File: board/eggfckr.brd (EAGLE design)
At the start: 114 x 77.5 mm, 22 parts, among them U1 ATTINY85-20PU, U2 ATTINY85-20PU, U3 ATTINY85-20PU, U4 ATTINY85-20PU

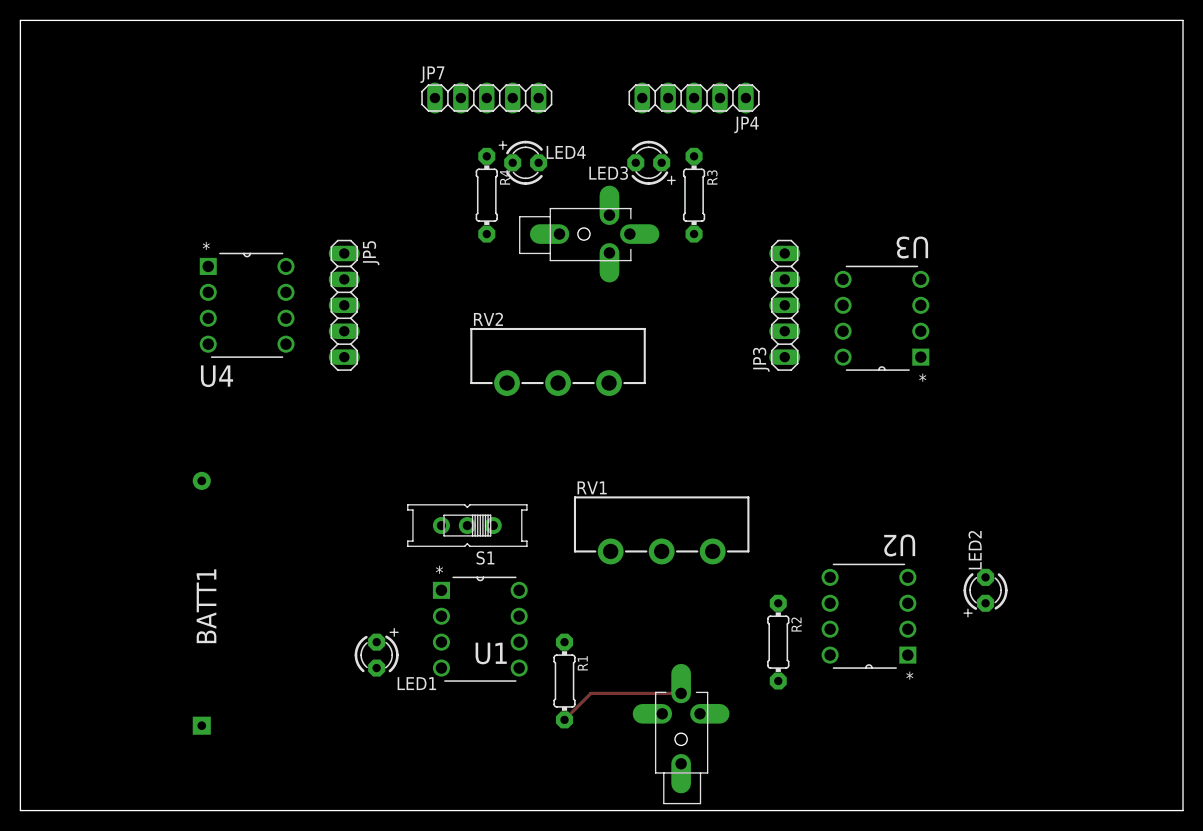
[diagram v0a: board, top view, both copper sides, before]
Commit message: getting ready for svg2snhn
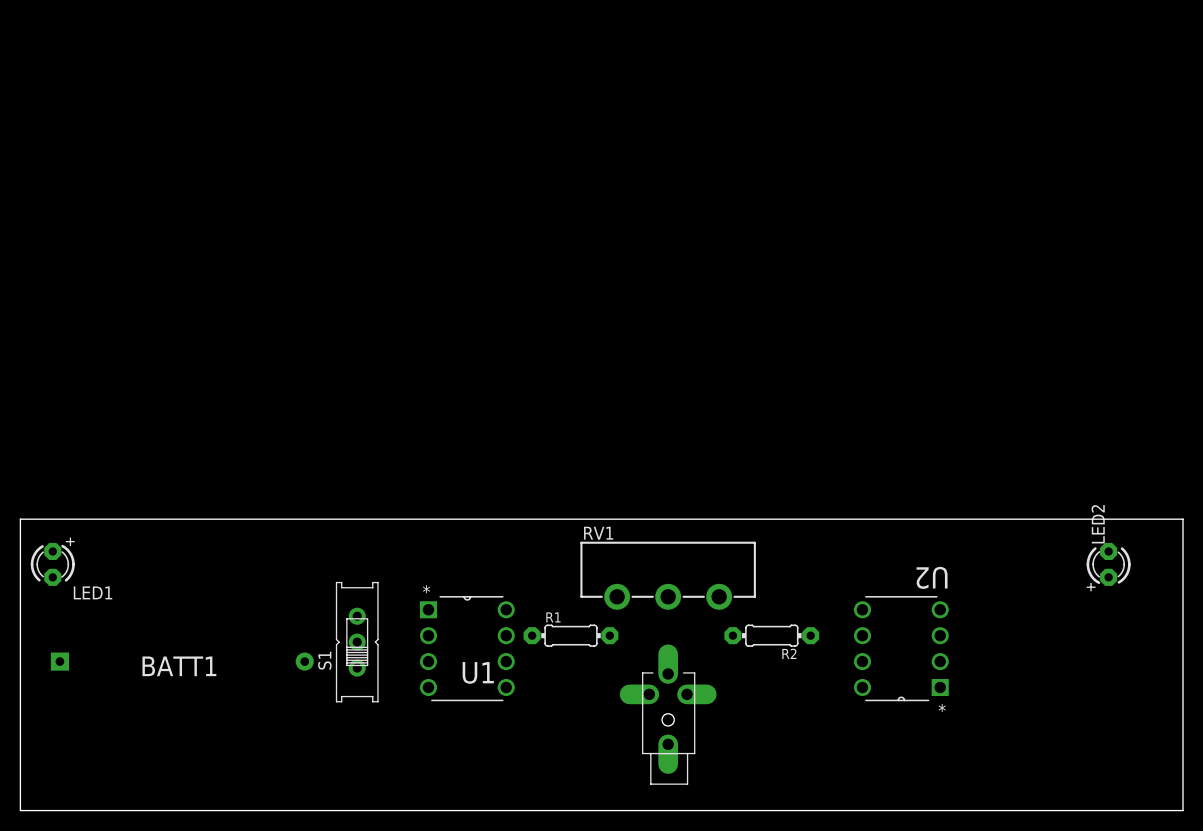
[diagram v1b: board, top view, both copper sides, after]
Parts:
- removed JP2: (no value), SparkFun-Connectors:STEREOJACK2.5MM_SPECIA_POGOPINS
- removed JP3, JP4, JP5, JP7: (no value), eggfckr:1X05
- removed LED3, LED4: (no value), adafruit:LED3MM
- removed R3, R4: (no value), adafruit:0204/7
- removed RV2: (no value), SparkFun-Electromechanical:POT_ALPHA_RV16AF-20
- removed U3, U4: ATTINY85-20PU, Atmel_By_element14_Batch_1-00:DIP254P762X533-8
- moved LED1 33.0 mm to (3.17, 24.1)
- moved S1 15.7 mm to (33.0, 16.5), turned to 90 degrees
- moved LED2 12.3 mm to (106.7, 24.1)
- moved BATT1 6.02 mm to (15.9, 14.6), turned to 180 degrees
- moved R1 4.49 mm to (54.0, 17.1), turned to 0 degrees
- moved RV1 4.49 mm to (63.5, 21.0)
- moved U2 4.49 mm to (82.5, 19.7)
- moved U1 2.29 mm to (47.6, 12.1)
- moved JP1 2.29 mm to (63.5, 8.89)
- moved R2 0.90 mm to (73.7, 17.1), turned to 180 degrees
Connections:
- removed net N$10: JP3.4, U3.3
- removed net N$11: JP4.2, JP7.2, RV2.2
- removed net N$12: JP7.3, R4.1
- removed net N$13: JP4.4, LED3.A
- removed net N$14: JP5.4, U4.3
- removed net N$15: JP2.SHIELD, R4.2
- removed net N$16: JP2.TIP, R3.2
- removed net N$17: JP3.1, U3.8
- removed net N$18: JP3.3, U3.6
- removed net N$19: JP3.2, U3.7
- removed net N$20: JP3.5, U3.4
- removed net N$21: JP5.1, U4.8
- removed net N$22: JP5.3, U4.6
- removed net N$23: JP5.2, U4.7
- removed net N$24: JP5.5, U4.4
- removed net N$30: JP7.4, LED4.A
- removed net N$9: JP4.3, R3.1
- net GND: no longer JP2.RING1, JP4.5, JP7.5, LED3.K, LED4.K, RV2.3
- net VCC: no longer JP4.1, JP7.1, RV2.1
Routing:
- net N$3: track 12.5 -> 0.00 mm
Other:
- board size 114 x 77.5 mm -> 114 x 28.6 mm
